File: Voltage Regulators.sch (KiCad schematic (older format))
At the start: 23 parts, among them P1 CONN_01X02, P3 CONN_01X02, U1 TS30042, U2 NCP700B, U3 MIC2288

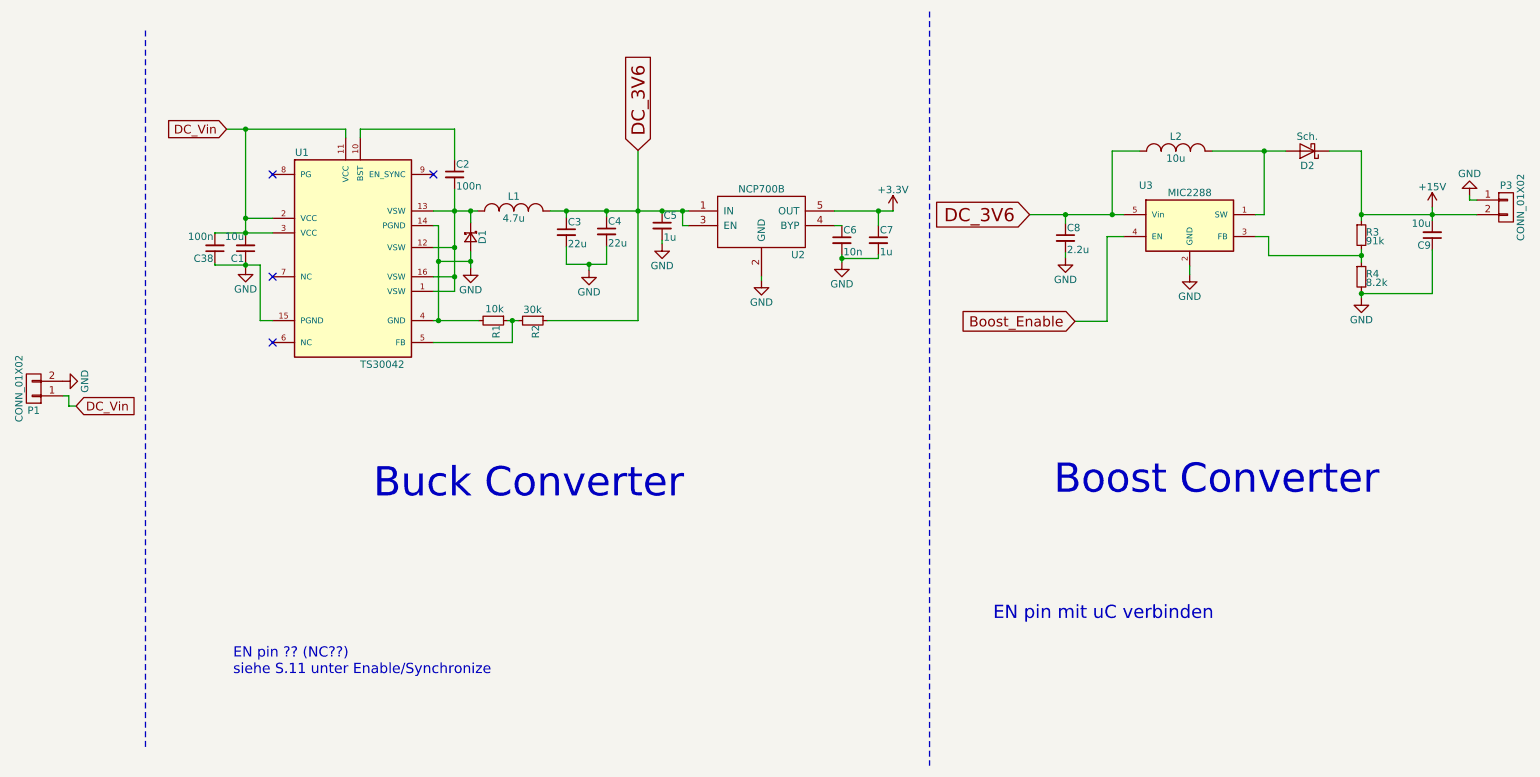
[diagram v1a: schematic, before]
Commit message: V1.0
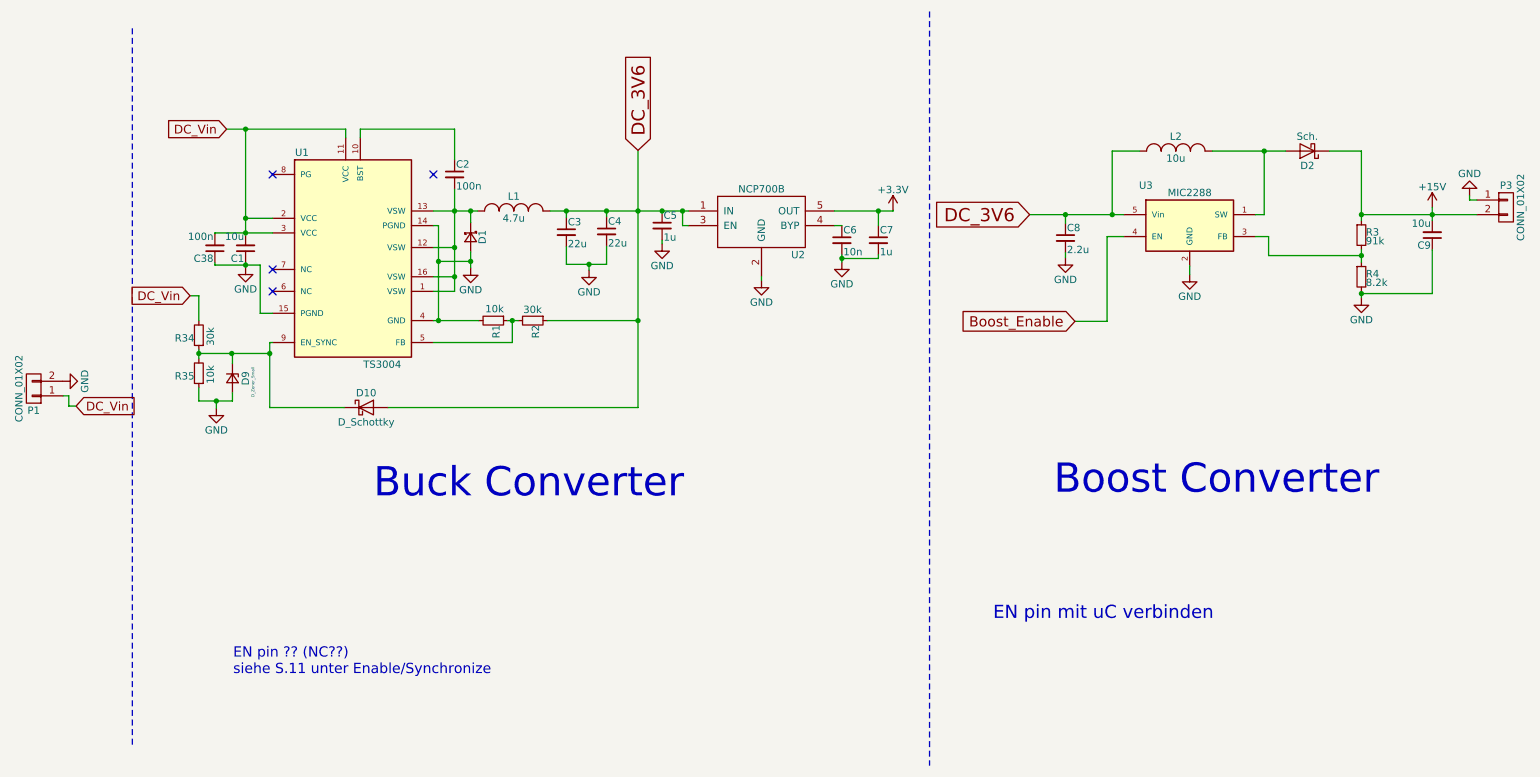
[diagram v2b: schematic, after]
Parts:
- removed U1: TS30042, Housings_DFN_QFN:QFN-16-1EP_3x3mm_Pitch0.5mm, symbol TS30042
- added D10: D_Schottky, .pretty:D_SOD-123, symbol D_Schottky
- added D9: D_Zener_Small, Diodes_SMD:D_SOD-323, symbol D_Zener_Small
- added R34: 30k, Resistors_SMD:R_0603, symbol R_Small
- added R35: 10k, Resistors_SMD:R_0603, symbol R_Small
- added U1: TS3004, Housings_DFN_QFN:QFN-16-1EP_3x3mm_Pitch0.5mm, symbol TS3004
- U3: footprint TO_SOT_Packages_SMD:TSOT-23-5 -> Footprints:TSOP-5
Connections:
- net DC_3V6: now also D10.2 (A)
- net DC_Vin: now also R34.2, U1.11 (VCC), U1.2 (VCC), U1.3 (VCC)
- net GND: now also D9.2 (A), R35.1, U1.14 (PGND), U1.15 (PGND), U1.4 (GND)
- net at C2.2, D1.1 (K), L1.1: now also U1.1 (VSW), U1.12 (VSW), U1.13 (VSW), U1.16 (VSW)
- net at C2.1: now also U1.10 (BST)
- net at R1.1, R2.2: now also U1.5 (FB)
- new net: D10.1 (K), D9.1 (K), R34.1, R35.2, U1.9 (EN_SYNC)
